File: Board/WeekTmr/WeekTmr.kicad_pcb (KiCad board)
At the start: 2 copper layers, 24 parts, among them J11 TMR1.1, J12 TMR1.2, J21 TMR2.1, J22 TMR2.2, J3 Barrel_Jack_MountingPin, J4 DS3231, K1 FINDER-40.52, K2 FINDER-40.52, Q1 BC817, Q2 BC817, SW1 DOWN_BUT, SW2 UP_BUT, SW3 SELECT_BUT, U1 NHD-0420H1Z

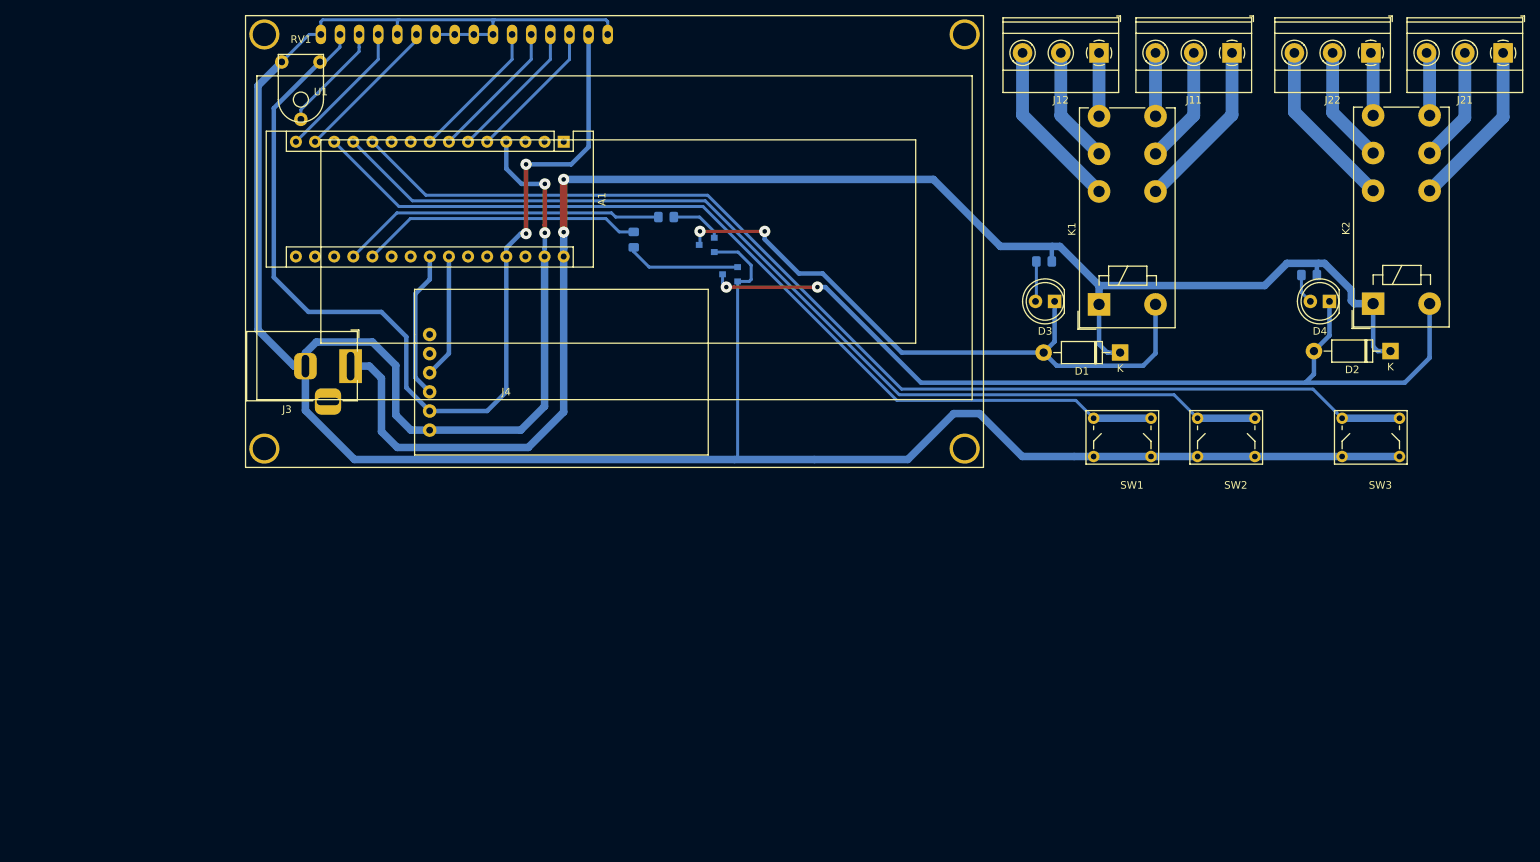
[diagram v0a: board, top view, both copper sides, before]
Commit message: board update
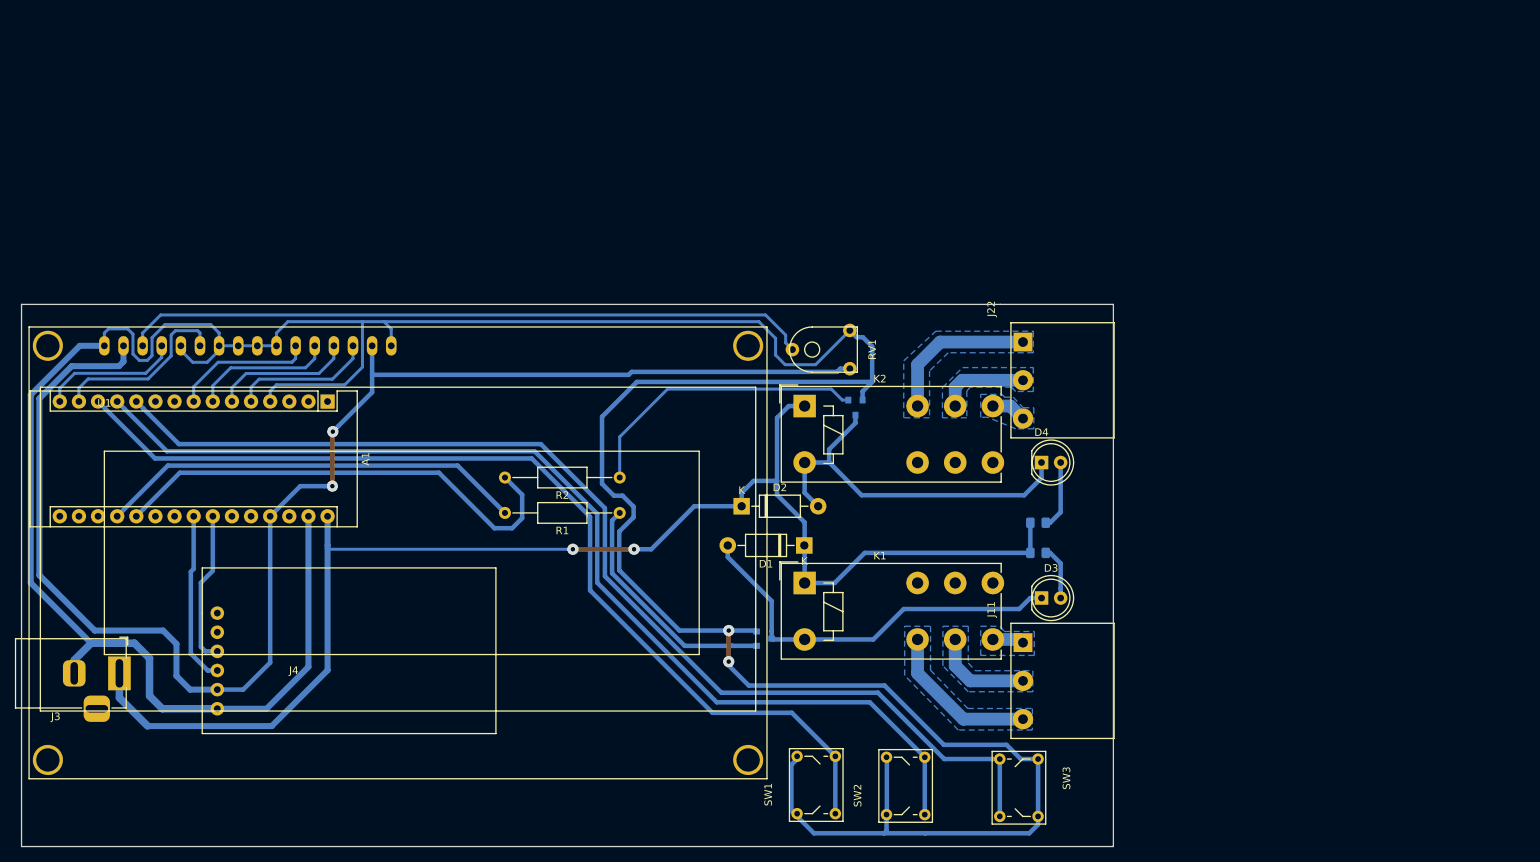
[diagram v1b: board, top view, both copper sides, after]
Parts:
- removed J12: TMR1.2, TerminalBlock_Phoenix:TerminalBlock_Phoenix_MKDS-1,5-3-5.08_1x03_P5.08mm_Horizontal
- removed J21: TMR2.1, TerminalBlock_Phoenix:TerminalBlock_Phoenix_MKDS-1,5-3-5.08_1x03_P5.08mm_Horizontal
- A1: footprint Module:Arduino_Nano -> KiCad_Library:Arduino_Nano_direct_Slot
- J11, J22: footprint TerminalBlock_Phoenix:TerminalBlock_Phoenix_MKDS-1,5-3-5.08_1x03_P5.08mm_Horizontal -> KiCad_Library:COMET_2EDGR-5.08-14-00AH
- R1, R2: footprint Resistor_SMD:R_0805_2012Metric_Pad1.15x1.40mm_HandSolder -> Resistor_THT:R_Axial_DIN0207_L6.3mm_D2.5mm_P15.24mm_Horizontal; moved to F.Cu
- moved D2 88.6 mm to (123.6, 94.8), turned to 0 degrees
- moved J11 87.9 mm to (161.0, 118.0), turned to 270 degrees
- moved RV1 82.3 mm to (138.0, 74.0), turned to 90 degrees
- moved K2 76.7 mm to (132.0, 81.5), turned to 0 degrees
- moved SW2 68.2 mm to (142.9, 135.8), turned to 90 degrees
- moved SW1 66.8 mm to (131.0, 135.6), turned to 90 degrees
- moved J22 63.4 mm to (161.0, 78.1), turned to 270 degrees
- moved SW3 62.6 mm to (163.0, 128.4), turned to 270 degrees
- moved K1 53.8 mm to (132.0, 105.0), turned to 0 degrees
- moved Q1 52.8 mm to (126.6, 112.4), turned to 0 degrees
- moved J3 51.1 mm to (41.0, 117.0)
- moved U1 50.4 mm to (29.0, 71.0)
- moved D1 49.1 mm to (132.0, 100.0)
- moved R4 48.8 mm to (163.0, 97.0), turned to 0 degrees
- moved A1 46.6 mm to (68.6, 80.9)
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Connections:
- J11 pad 1: NC1.1 -> NO1.1
- J11 pad 3: NO1.1 -> NC1.1
- J22 pad 1: NO2.2 -> NC2.2
- J22 pad 3: NC2.2 -> NO2.2
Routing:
- net GND: track 380.5 -> 467.2 mm
- net Net-(RV1-Pad2): track 14.5 -> 91.5 mm
- net Net-(D2-Pad2): track 121.3 -> 50.6 mm, vias 2 -> 0
- net +5V: track 135.5 -> 193.6 mm
- net Net-(D1-Pad2): track 84.9 -> 53.0 mm, vias 2 -> 0
- net +12V: track 210.4 -> 184.1 mm
- net tmr2_out: track 37.5 -> 63.6 mm
- net Net-(Q1-Pad1): track 6.98 -> 31.6 mm
- net Net-(Q2-Pad1): track 15.2 -> 39.0 mm
- net NC1.2: track 22.6 -> 0.00 mm
- net NC2.1: track 22.3 -> 0.00 mm
- net COM1.2: track 15.5 -> 0.00 mm
- net COM2.1: track 15.2 -> 0.00 mm
- net tmr1_out: track 43.1 -> 56.9 mm
- net NO2.1: track 8.47 -> 0.00 mm
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- added copper zone on B.Cu, net COM1.1
- added copper zone on B.Cu, net COM2.2
- added copper zone on B.Cu, net NC1.1
- added copper zone on B.Cu, net NC2.2
- added copper zone on B.Cu, net NO1.1
- added copper zone on B.Cu, net NO2.2
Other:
- board outline added: 145 x 72 mm
